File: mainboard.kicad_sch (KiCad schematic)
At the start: 27 parts, among them U1 LIS2DW12, U2 AP2205-3.0, U3 BQ21080, U4 STM32L412KBTx

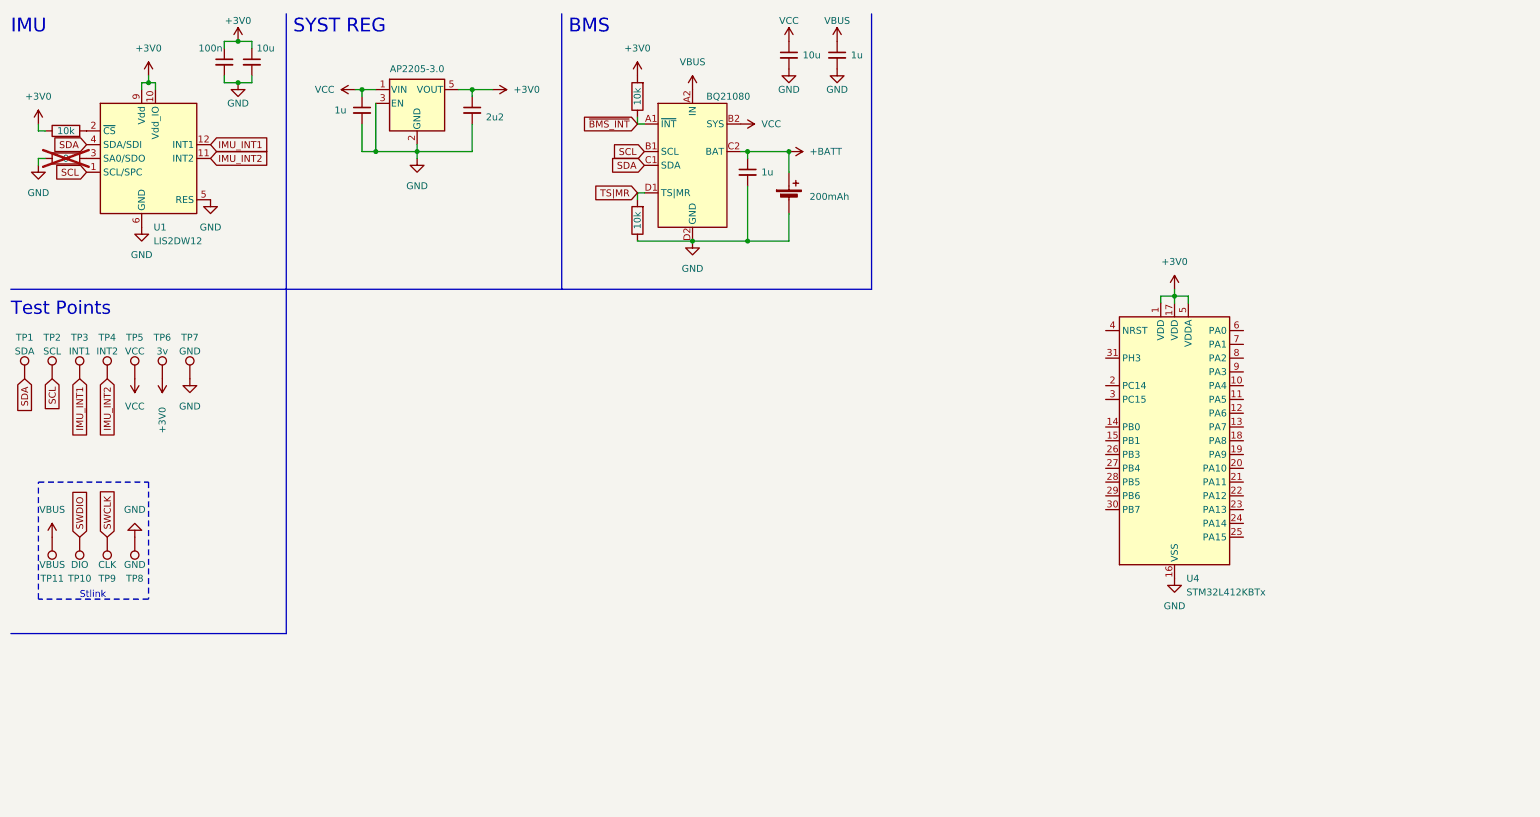
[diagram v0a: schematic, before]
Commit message: Diode layout, majority of schema, tile thoughts
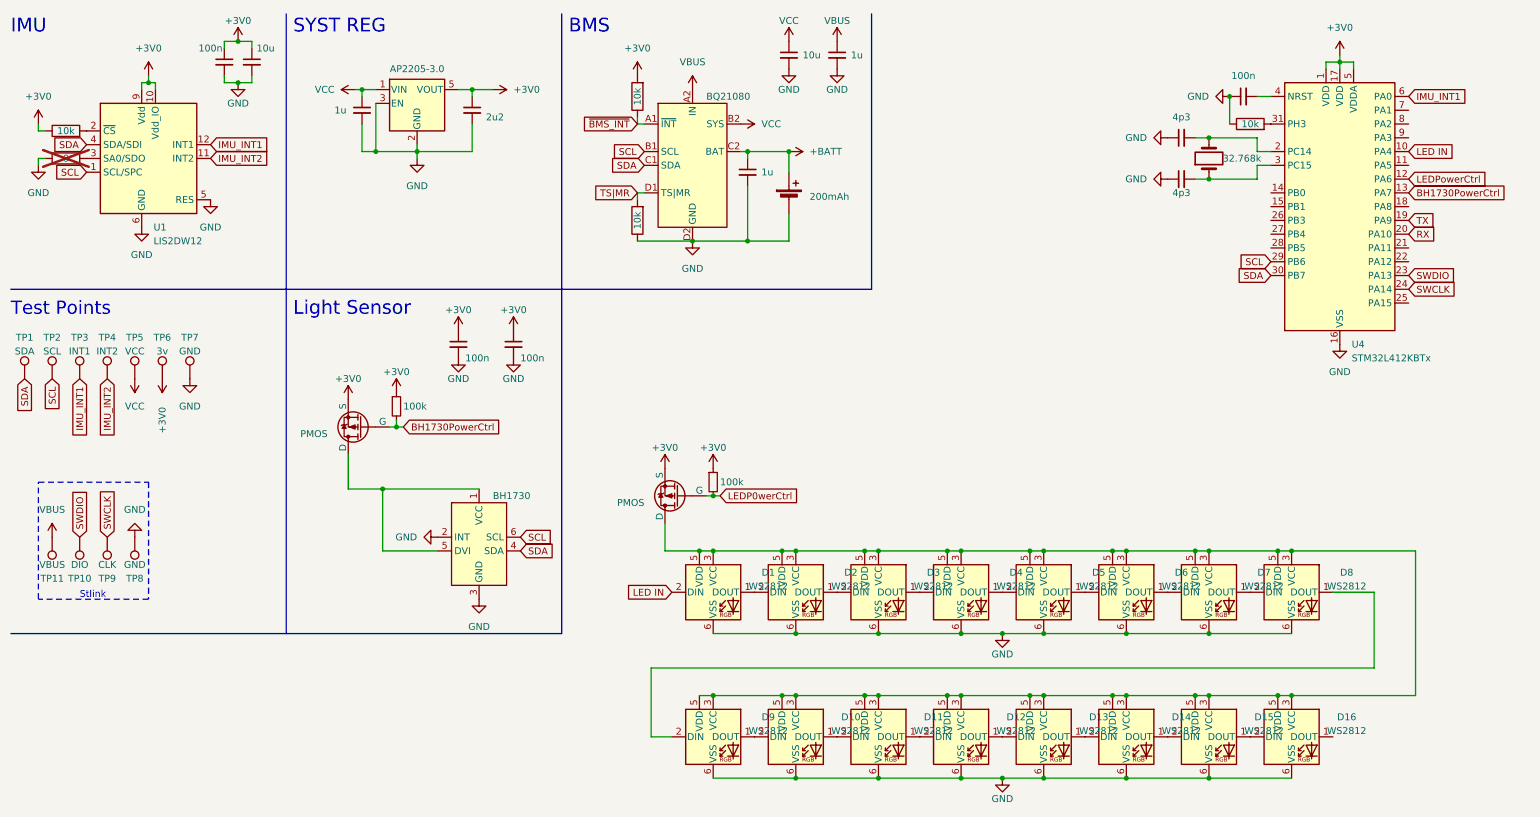
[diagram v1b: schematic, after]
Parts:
- added C10, C8, C9: 100n, Capacitor_SMD:C_0402_1005Metric, symbol Device:C_Small
- added C11, C12: 4p3, Capacitor_SMD:C_0402_1005Metric, symbol Device:C_Small
- added D1, D10, D11, D12, D13, D14, D15, D16, D2, D3, D4, D5, D6, D7, D8, D9: WS2812, LED_SMD:LED_WS2812_PLCC6_5.0x5.0mm_P1.6mm, symbol LED:WS2812
- added Q1, Q2: PMOS, Package_TO_SOT_SMD:SOT-23-3, symbol Simulation_SPICE:PMOS
- added R5, R7: 100k, Resistor_SMD:R_0402_1005Metric, symbol Device:R_Small
- added R6: 10k, Resistor_SMD:R_0402_1005Metric, symbol Device:R
- added U5: BH1730, symbol Components:BH1730
- added Y1: 32.768k, Crystal:Crystal_SMD_5032-2Pin_5.0x3.2mm, symbol Device:Crystal
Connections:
- net +3V0: now also C8.1, C9.1, Q1.3 (S), Q2.3 (S), R5.1, R7.1
- net GND: now also C10.1, C11.1, C12.1, C8.2, C9.2, D1.6 (VSS), D10.6 (VSS), D11.6 (VSS), D12.6 (VSS), D13.6 (VSS), D14.6 (VSS), D15.6 (VSS), D16.6 (VSS), D2.6 (VSS), D3.6 (VSS), D4.6 (VSS), D5.6 (VSS), D6.6 (VSS), D7.6 (VSS), D8.6 (VSS), D9.6 (VSS), R6.1, U5.2 (INT), U5.3 (GND)
- net IMU_INT1: now also U4.6 (PA0)
- net SCL: now also U4.29 (PB6), U5.6 (SCL)
- net SDA: now also U4.30 (PB7), U5.4 (SDA)
- net SWCLK: now also U4.24 (PA14)
- net SWDIO: now also U4.23 (PA13)
- net LED IN: now reaches U4.10 (PA4)
- net LED IN: now also D1.2 (DIN)
- net LEDPowerCtrl: now reaches U4.12 (PA6)
- net BH1730PowerCtrl: now reaches U4.13 (PA7)
- net BH1730PowerCtrl: now also Q1.2 (G), R5.2
- net TX: now reaches U4.19 (PA9)
- net at U4.2 (PC14): now also C11.2, Y1.2
- net RX: now reaches U4.20 (PA10)
- net at U4.3 (PC15): now also C12.2, Y1.1
- net at U4.31 (PH3): now also R6.2
- net at U4.4 (NRST): now also C10.2
- new net: D12.1 (DOUT), D13.2 (DIN)
- new net: D11.1 (DOUT), D12.2 (DIN)
- new net: D1.3 (VCC), D1.5 (VDD), D10.3 (VCC), D10.5 (VDD), D11.3 (VCC), D11.5 (VDD), D12.3 (VCC), D12.5 (VDD), D13.3 (VCC), D13.5 (VDD), D14.3 (VCC), D14.5 (VDD), D15.3 (VCC), D15.5 (VDD), D16.3 (VCC), D16.5 (VDD), D2.3 (VCC), D2.5 (VDD), D3.3 (VCC), D3.5 (VDD), D4.3 (VCC), D4.5 (VDD), D5.3 (VCC), D5.5 (VDD), D6.3 (VCC), D6.5 (VDD), D7.3 (VCC), D7.5 (VDD), D8.3 (VCC), D8.5 (VDD), D9.3 (VCC), D9.5 (VDD), Q2.1 (D)
- new net: D3.1 (DOUT), D4.2 (DIN)
- new net: D2.1 (DOUT), D3.2 (DIN)
- new net: D14.1 (DOUT), D15.2 (DIN)
- new net: D13.1 (DOUT), D14.2 (DIN)
- new net: D5.1 (DOUT), D6.2 (DIN)
- new net: D4.1 (DOUT), D5.2 (DIN)
- new net: D10.1 (DOUT), D11.2 (DIN)
- new net: D10.2 (DIN), D9.1 (DOUT)
- new net: D8.1 (DOUT), D9.2 (DIN)
- new net: D7.1 (DOUT), D8.2 (DIN)
- new net: Q1.1 (D), U5.1 (VCC), U5.5 (DVI)
- new net: D1.1 (DOUT), D2.2 (DIN)
- new net: D6.1 (DOUT), D7.2 (DIN)
- new net: D15.1 (DOUT), D16.2 (DIN)
- new net LEDP0werCtrl: Q2.2 (G), R7.2
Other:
- note added: "Light Sensor"
- moved on the sheet: U4
